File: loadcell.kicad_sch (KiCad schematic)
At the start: 5 parts, among them IC4 ADS131M02IRUKR, J4 B4B-XH-A_LF__SN_

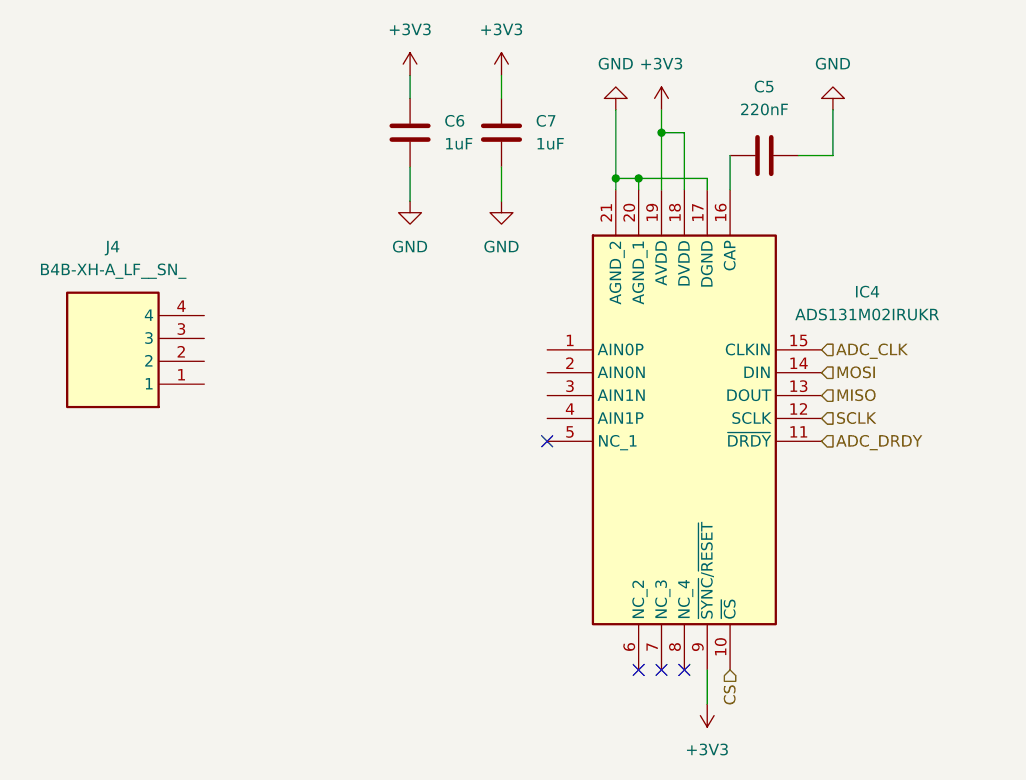
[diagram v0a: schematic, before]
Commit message: Added stuff
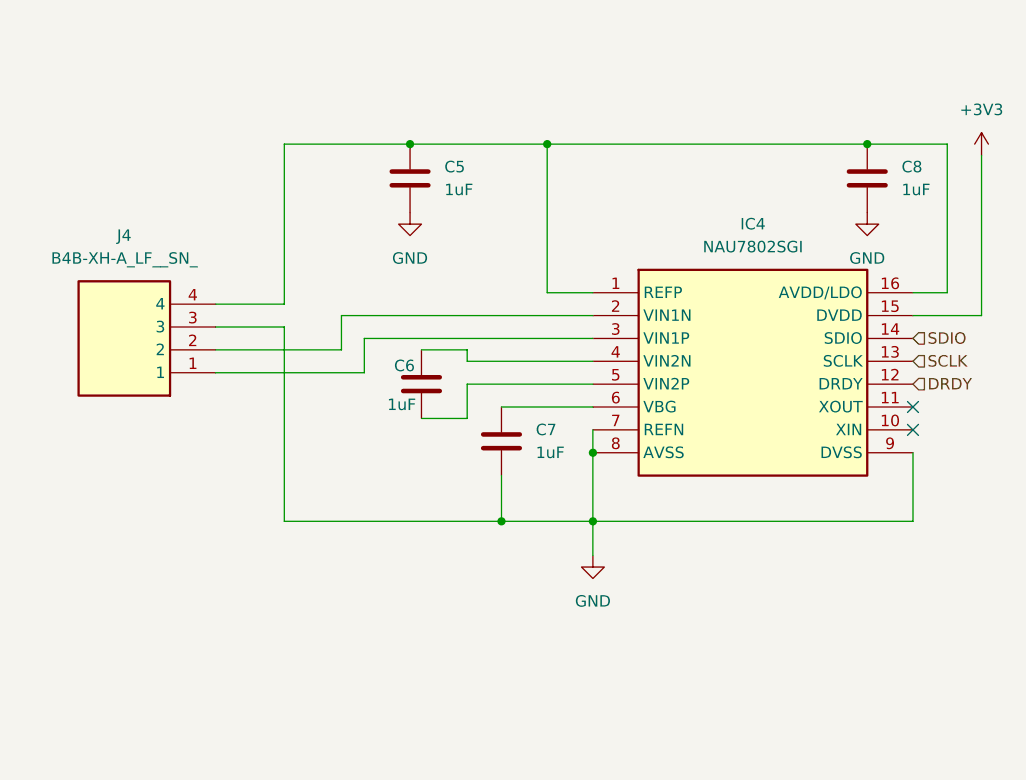
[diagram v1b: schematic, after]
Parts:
- removed IC4: ADS131M02IRUKR, QFN40P300X300X80-21N-D, symbol ADS131M02IRUKR:ADS131M02IRUKR
- added C8: 1uF, Capacitor_SMD:C_0402_1005Metric, symbol Device:C
- added IC4: NAU7802SGI, SOIC127P600X175-16N, symbol NAU7802SGI:NAU7802SGI
- C5: value 220nF -> 1uF
- C6, C7: footprint (none) -> Capacitor_SMD:C_0402_1005Metric
- J4: footprint B4BXHALFSN -> Library:B4BXHALFSN
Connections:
- net +3V3: now also IC4.15 (DVDD); no longer C6.1, C7.1
- net GND: now also J4.3, C8.2, IC4.7 (REFN), IC4.8 (AVSS), IC4.9 (DVSS); no longer C6.2
- net SCLK: now also IC4.13 (SCLK)
- net at C5.1: now also J4.4, C8.1, IC4.1 (REFP), IC4.16 (AVDD/LDO)
- net at J4.1: now also IC4.3 (VIN1P)
- net at J4.2: now also IC4.2 (VIN1N)
- new net: C6.1, IC4.4 (VIN2N)
- new net: C6.2, IC4.5 (VIN2P)
- new net: C7.1, IC4.6 (VBG)
- new net DRDY: IC4.12 (DRDY)
- new net SDIO: IC4.14 (SDIO)
- no-connect marks 4 -> 2
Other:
- moved on the sheet: J4
